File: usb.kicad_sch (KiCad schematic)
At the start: 5 parts, among them J201 USB_C_Receptacle_USB2.0_14P, U201 SLLC23T5V2U

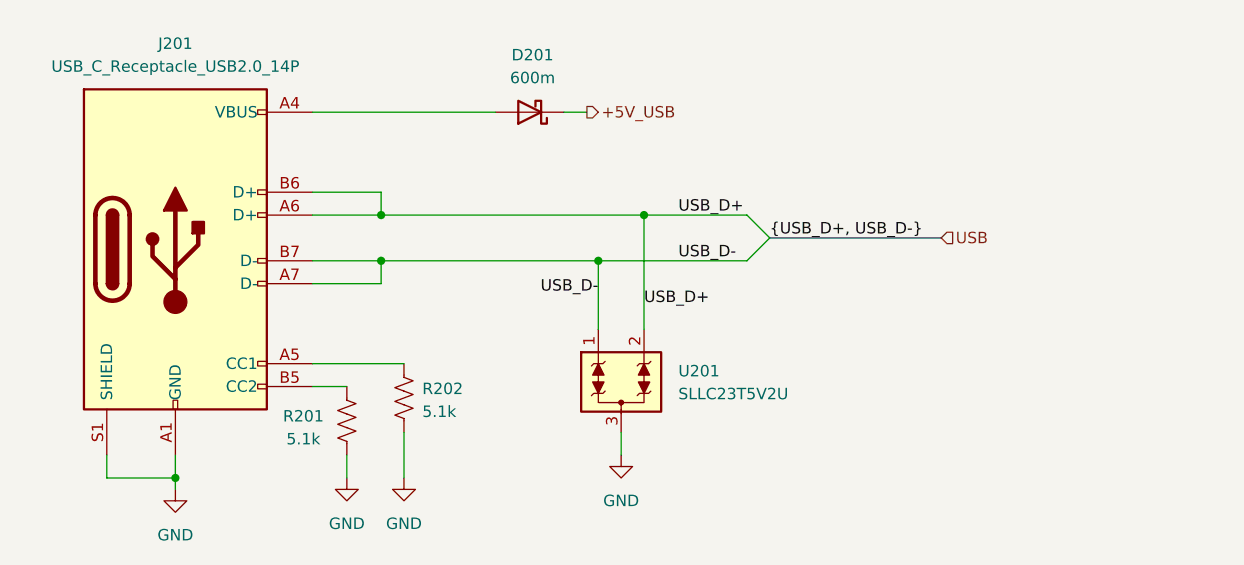
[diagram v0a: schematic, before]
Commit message: updated layout (usb/buttons), generated gerbers
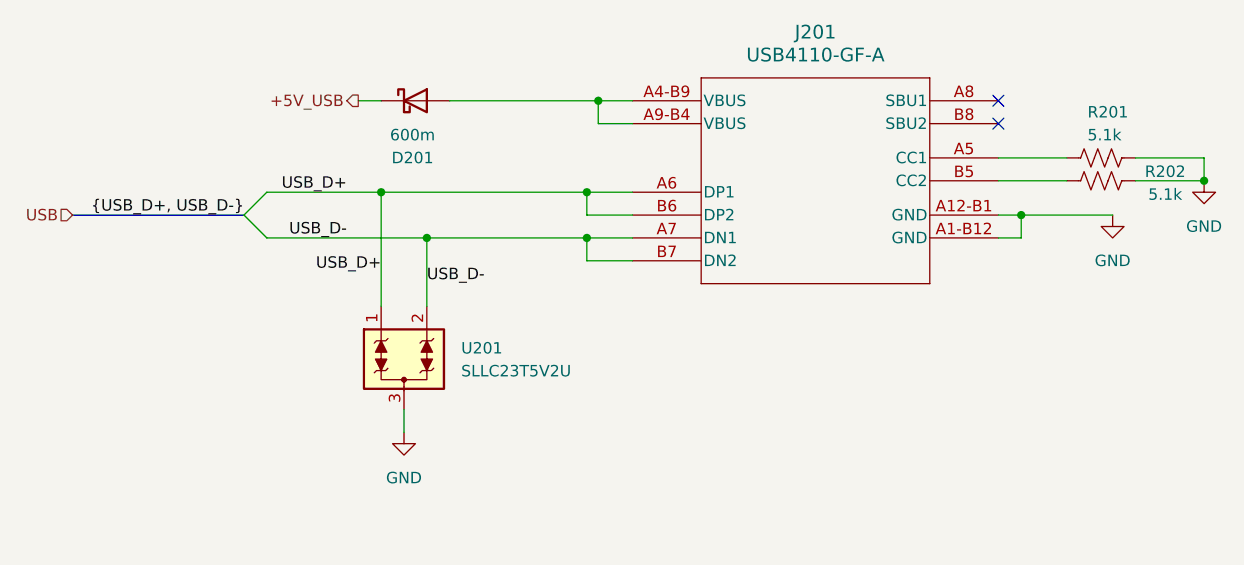
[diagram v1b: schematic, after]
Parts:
- removed J201: USB_C_Receptacle_USB2.0_14P, Connector_USB:USB_C_Receptacle_G-Switch_GT-USB-7010ASV, symbol bfr_connectors:USB_C_Receptacle_USB2.0_14P
- added J201: USB4110-GF-A, USB4110_GF_A:USB4110-GF-A_GCT, symbol USB4110_GF_A:USB4110-GF-A
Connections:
- net GND: now also J201.A1-B12 (GND), J201.A12-B1 (GND)
- net USB_D+: now also U201.1, J201.A6 (DP1), J201.B6 (DP2); no longer U201.2
- net USB_D-: now also U201.2, J201.A7 (DN1), J201.B7 (DN2); no longer U201.1
- net at D201.2 (A): now also J201.A4-B9 (VBUS), J201.A9-B4 (VBUS)
- net at R202.2: now also J201.B5 (CC2)
- net at R201.2: now also J201.A5 (CC1)
- no-connect marks 0 -> 2
